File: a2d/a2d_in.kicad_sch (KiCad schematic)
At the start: 12 parts, among them U1 B3B-XH-A(LF)(SN), U2 2060-453/998-404

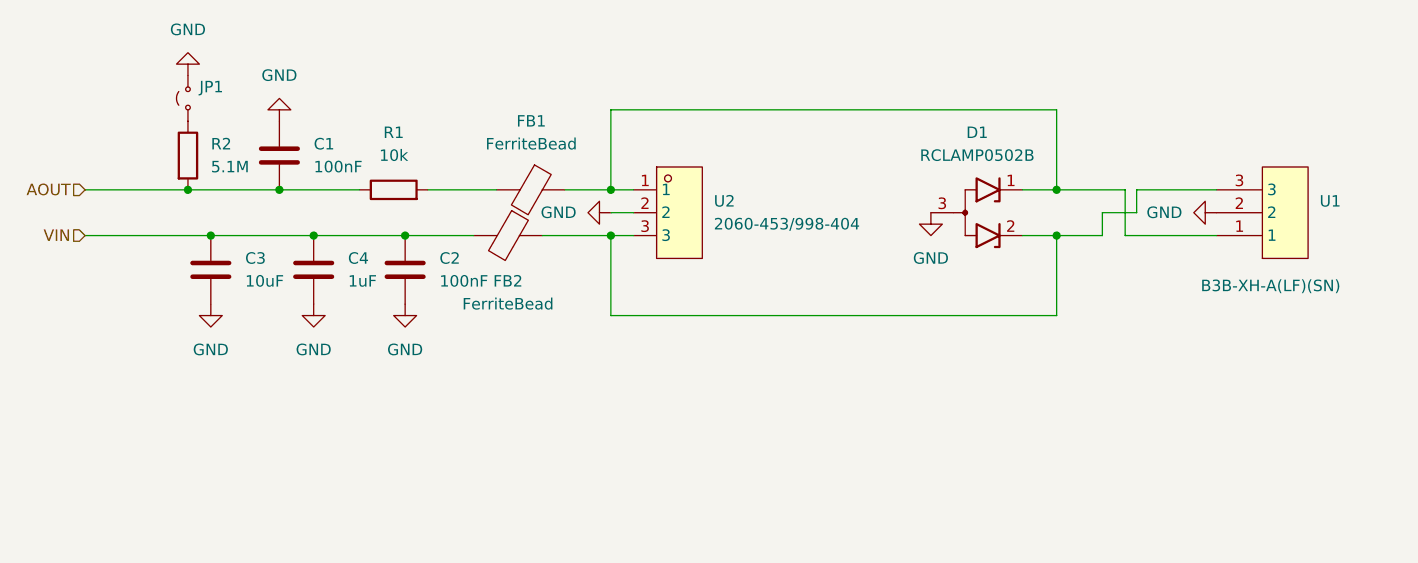
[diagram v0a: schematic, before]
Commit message: a2d v0.4
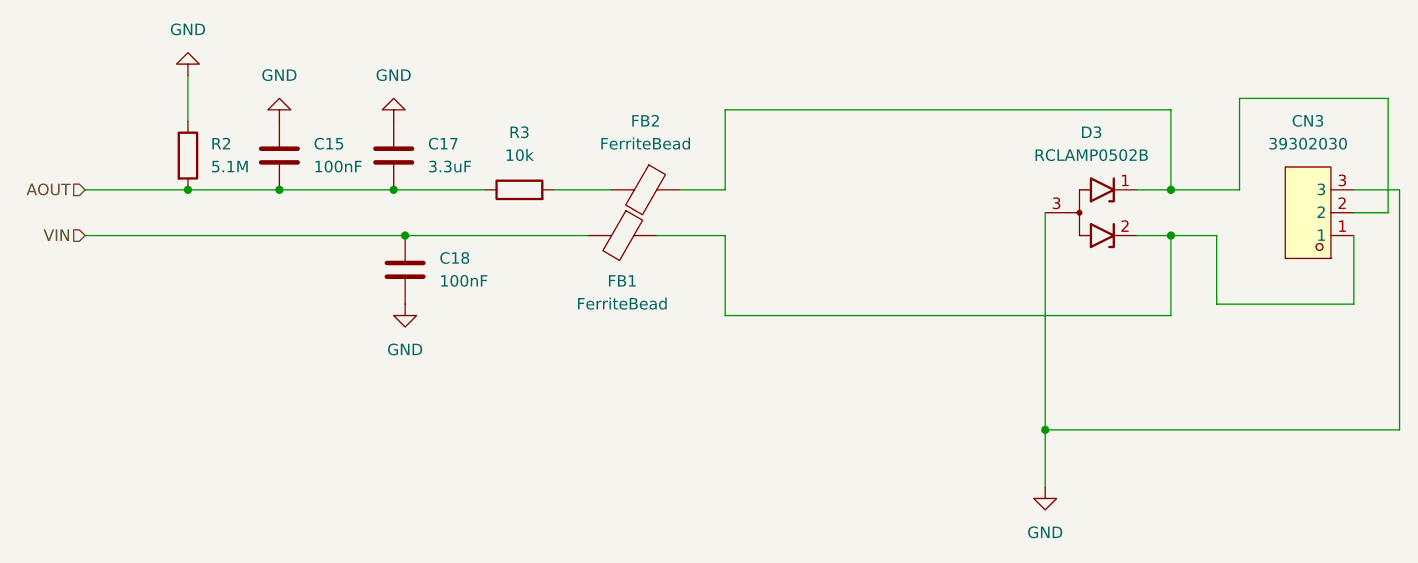
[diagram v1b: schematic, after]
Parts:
- removed C3: 10uF, Capacitor_SMD:C_0603_1608Metric, symbol Device:C
- removed C4: 1uF, Capacitor_SMD:C_0603_1608Metric, symbol Device:C
- removed JP1: Jumper_2_Small_Open, Connector_PinHeader_2.54mm:PinHeader_1x02_P2.54mm_Vertical, symbol Jumper:Jumper_2_Small_Open
- removed U1: B3B-XH-A(LF)(SN), easyeda2kicad:CONN-TH_3P-P2.50_A2501WV2-3P, symbol easyeda2kicad:B3B-XH-A(LF)(SN)
- removed U2: 2060-453/998-404, easyeda2kicad:CONN-SMD_2060-453, symbol easyeda2kicad:2060-453_998-404
- added C17: 3.3uF, Capacitor_SMD:C_0603_1608Metric, symbol Device:C
- added CN3: 39302030, easyeda2kicad:CONN-TH_3P-P4.20_39302030, symbol easyeda2kicad:39302030
- renumbered C1 to C15, C2 to C18, D1 to D3, FB2 to FB1, FB1 to FB2, R1 to R3
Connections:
- net AOUT: now also C17.2
- net GND: now also R2.1, C17.1, CN3.3
- net at D3.1 (K1), FB2.1: now also CN3.2
- net at D3.2 (K2), FB1.1: now also CN3.1
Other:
- moved on the sheet: D3, FB1, FB2, R3
